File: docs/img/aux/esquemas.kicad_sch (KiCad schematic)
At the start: 27 parts

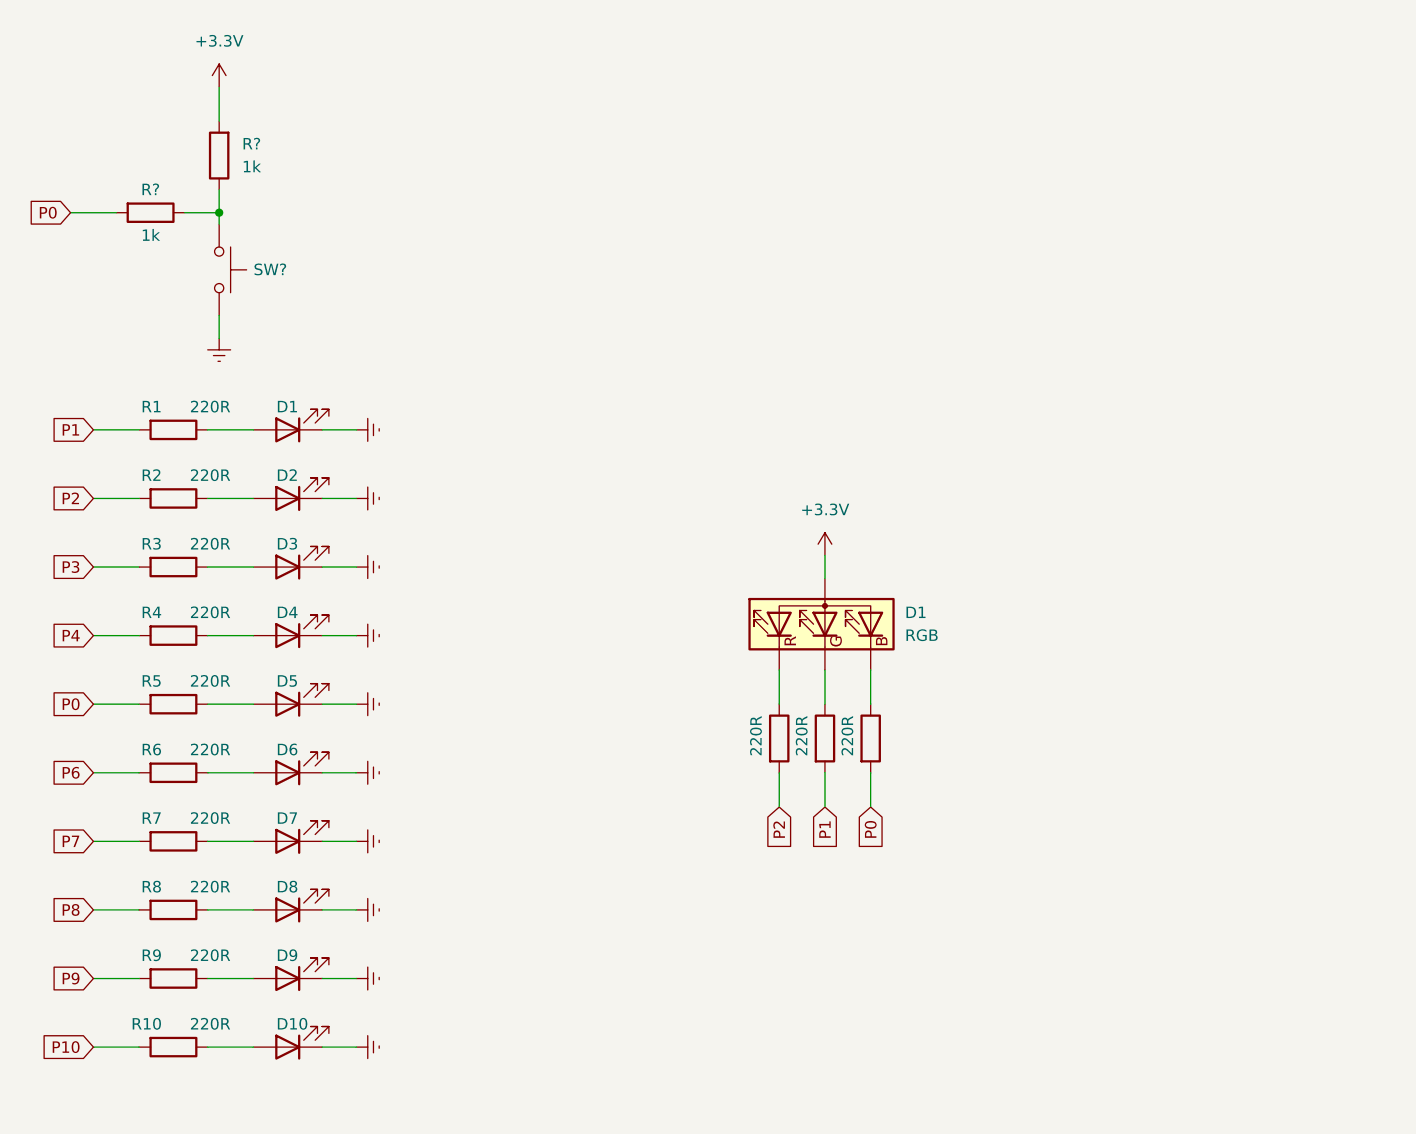
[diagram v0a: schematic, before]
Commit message: Hasta A14 incluida
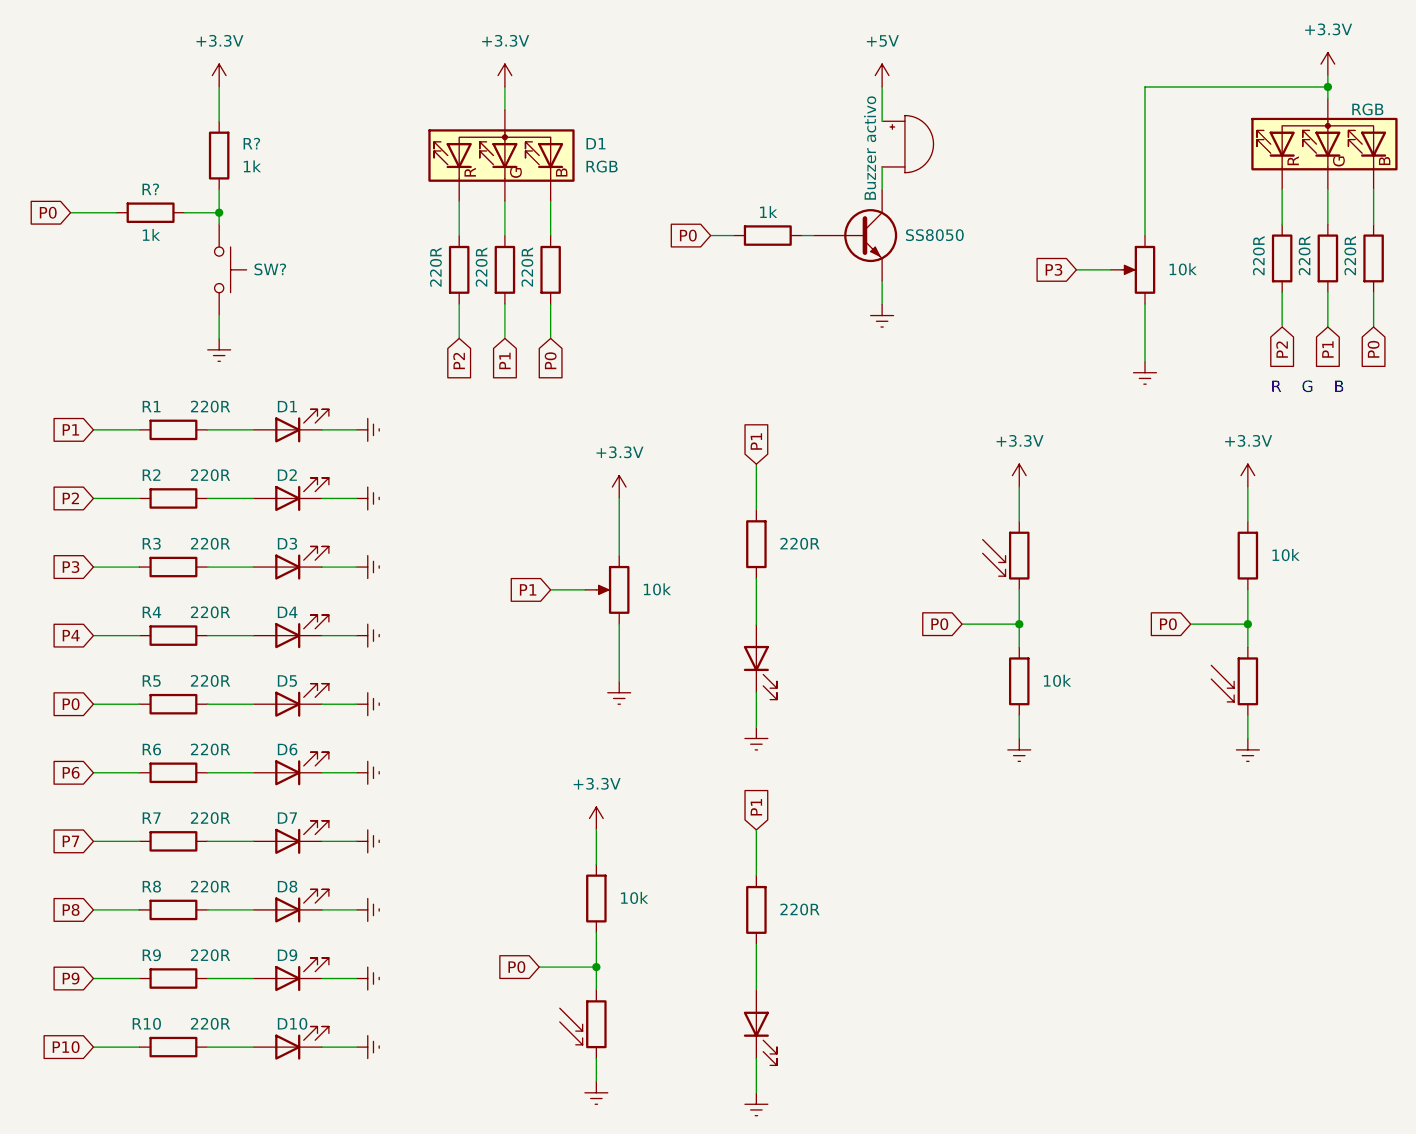
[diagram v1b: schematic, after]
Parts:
- added BZ?: Buzzer activo, symbol Device:Buzzer
- added D? (x2): LED, symbol Device:LED
- added D?: RGB, symbol Device:LED_RGBA
- added Q?: SS8050, Package_TO_SOT_THT:TO-92_Inline, symbol Transistor_BJT:2N3904
- added R? (x5): 220R, symbol Device:R
- added R? (x3): 10k, symbol Device:R
- added R?: 1k, symbol Device:R
- added R? (x3): R_Photo, symbol Device:R_Photo
- added RV? (x2): 10k, symbol Device:R_Potentiometer
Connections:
- net +3.3V: now also D?.4 (A), R?.1, R?.2, R?.2, RV?.1, RV?.1
- net GNDREF: now also D?.1 (K), D?.1 (K), Q?.1 (E), R?.1, R?.2, R?.2, RV?.3, RV?.3
- net P0: now also R?.1, R?.1, R?.1, R?.1, R?.2, R?.2, R?.2, R?.2
- net P1: now also R?.2, R?.2, R?.2, RV?.2
- net P2: now also R?.2
- net P3: now also RV?.2
- new net: D?.1 (RK), R?.1
- new net: D?.3 (BK), R?.1
- new net: D?.2 (A), R?.1 (x2)
- new net: D?.2 (GK), R?.1
- new net: Q?.2 (B), R?.1
- new net: BZ?.2 (+), Q?.3 (C)
- new net +5V: BZ?.1 (-)
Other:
- note added: "R G B"
- moved on the sheet: D1
